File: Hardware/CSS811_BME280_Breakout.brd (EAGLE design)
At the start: 25.4 x 25.4 mm, 25 parts, among them J1 JST, J2 CCS811 Options, J3 JST, J4 PTH, U2 CCS811

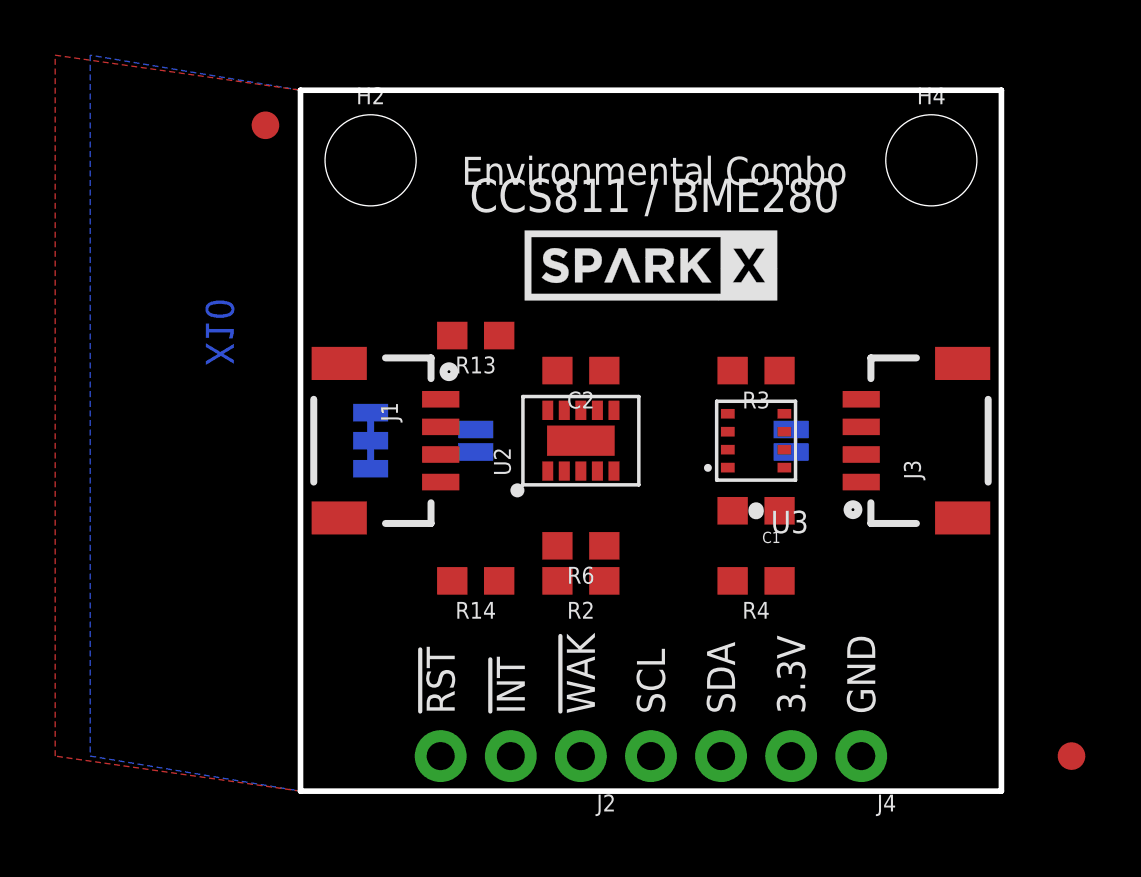
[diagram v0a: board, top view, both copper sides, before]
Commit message: Initial Layout Finished - Ready for Review
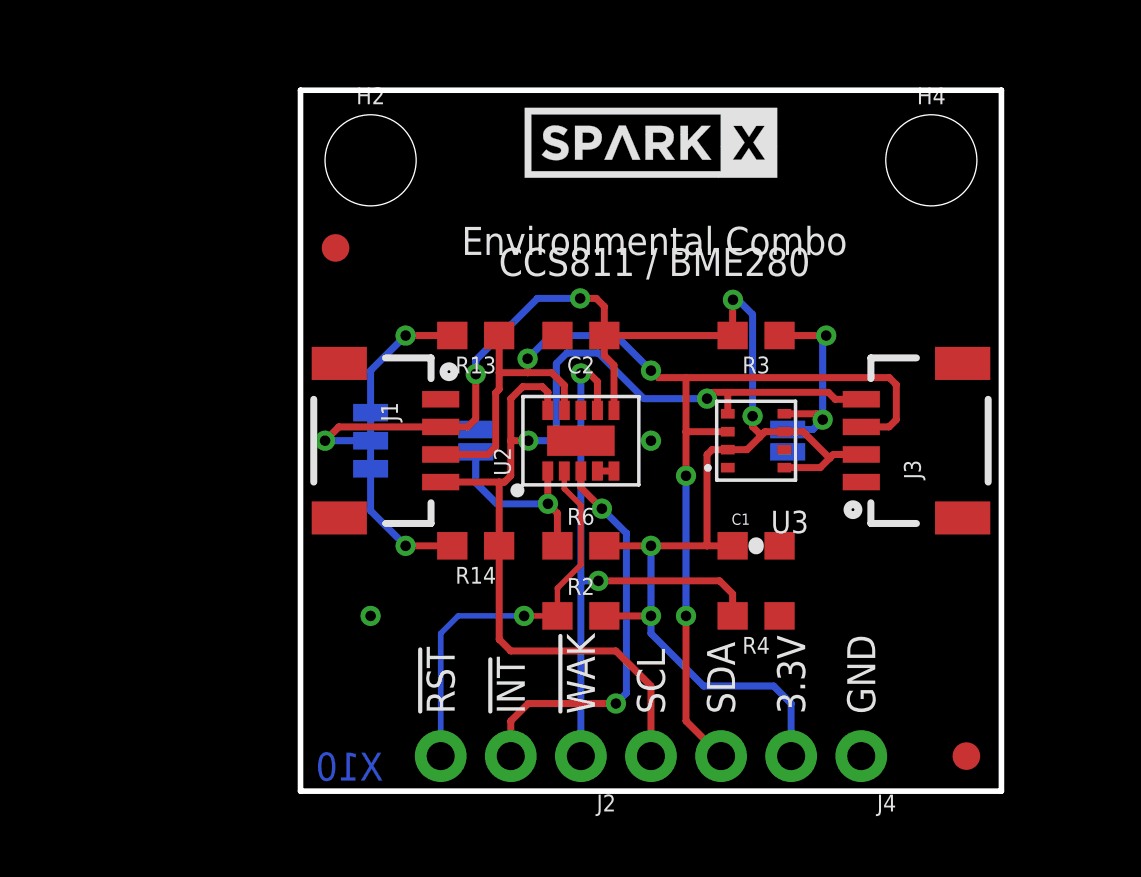
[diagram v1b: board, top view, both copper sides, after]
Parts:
- moved FD1 5.12 mm to (1.27, 19.7)
- moved U$1 4.45 mm to (12.7, 23.5)
- moved U$2 4.45 mm to (12.7, 23.5)
- moved FD2 3.81 mm to (24.1, 1.27)
- moved C2 1.27 mm to (10.2, 16.5)
- moved R3 1.27 mm to (16.5, 16.5)
- moved R14 1.27 mm to (6.35, 8.89)
- moved R2 1.27 mm to (10.2, 6.35), turned to 0 degrees
- moved R4 1.27 mm to (16.5, 6.35)
- moved C1 1.27 mm to (16.5, 8.89), turned to 0 degrees
- moved ADR2 0.13 mm to (17.7, 12.7)
- turned R6 to 0 degrees
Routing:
- net 3.3V: track 0.00 -> 59.6 mm, vias 0 -> 7
- net SDA: track 0.00 -> 43.0 mm, vias 0 -> 4
- net SCL: track 0.00 -> 39.3 mm, vias 0 -> 2
- net !WAKE: track 0.00 -> 22.4 mm, vias 0 -> 2
- net !RST: track 0.00 -> 14.8 mm, vias 0 -> 1
- net !INT: track 0.00 -> 14.6 mm, vias 0 -> 2
- net SDO/ADR: track 0.00 -> 7.68 mm, vias 0 -> 2
- net CCS811_ADDR: track 0.00 -> 6.90 mm, vias 0 -> 1
- net N$4: track 0.00 -> 5.01 mm, vias 0 -> 1
- net N$5: track 0.00 -> 5.01 mm, vias 0 -> 1
- net NTC_SENSE: track 0.00 -> 0.60 mm
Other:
- board text added: "ADR2"
